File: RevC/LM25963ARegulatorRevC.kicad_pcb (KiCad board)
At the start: 2 copper layers, 61.2 x 24.6 mm, 18 parts, among them U1 LM2596S-ADJ

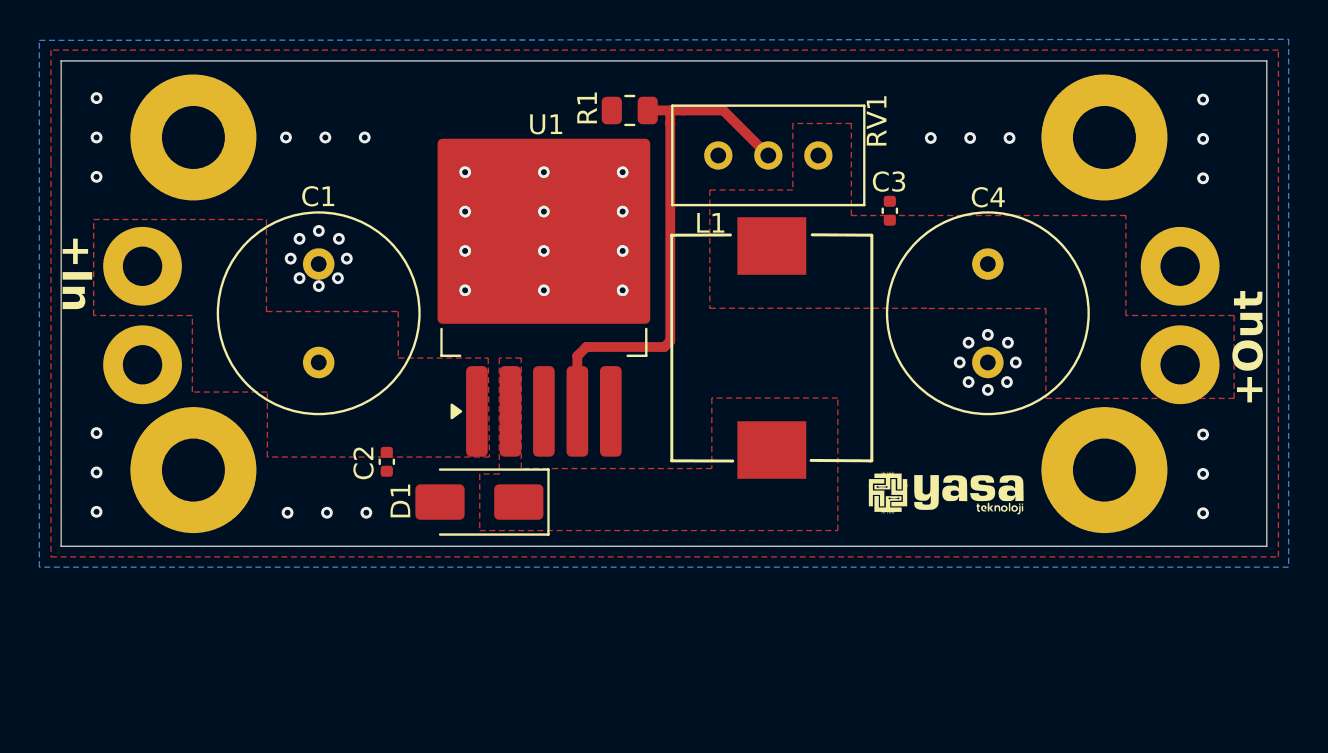
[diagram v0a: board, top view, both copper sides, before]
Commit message: Add files via upload
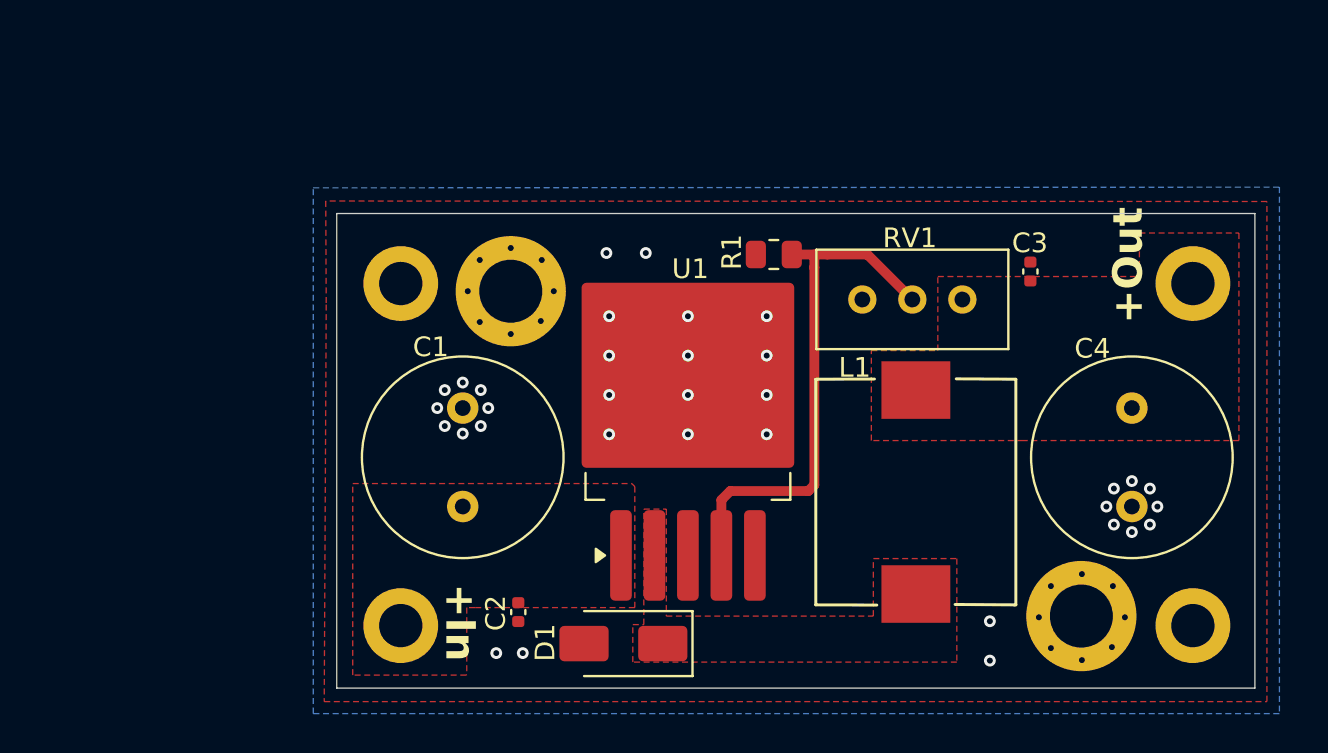
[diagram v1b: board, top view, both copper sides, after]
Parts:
- removed the ? at (121.1, 107.9)
- removed the ? at (167.4, 91.0)
- removed the ? at (167.4, 107.9)
- removed the ? at (171.3, 97.5)
- removed the ? at (171.3, 102.5)
- removed the REF** at (121.1, 91.0)
- removed the REF** at (118.6, 97.5)
- removed the REF** at (118.6, 102.5)
- added ?: , , F.Cu at (137.3, 98.8)
- added ?: , , F.Cu at (171.9, 98.4)
- added ?: , , F.Cu at (131.7, 98.4)
- added ?: , , F.Cu at (171.9, 115.8)
- added REF**: MountingHole_2.2mm_M2_DIN965_Pad, MountingHole:MountingHole_2.2mm_M2_DIN965_Pad, F.Cu at (131.7, 115.8)
- added REF**: MountingHole_3.2mm_M3_DIN965_Pad, MountingHole:MountingHole_3.2mm_M3_DIN965_Pad, F.Cu at (166.2, 115.3)
- G***: moved to B.Cu
- moved U1 10.3 mm to (146.3, 104.6)
- moved C1 10.3 mm to (134.8, 109.8)
- moved C4 10.3 mm to (168.8, 104.8)
- moved R1 10.3 mm to (150.6, 97.0)
- moved RV1 10.3 mm to (155.1, 99.2)
- moved L1 10.3 mm to (157.8, 109.0)
- moved D1 10.3 mm to (143.0, 116.7)
- moved C2 10.1 mm to (137.6, 115.1)
- moved G*** 8.23 mm to (151.1, 108.7)
- moved C3 7.78 mm to (163.7, 97.8)
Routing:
- net GND: vias 49 -> 50
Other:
- board size 61.2 x 24.6 mm -> 46.6 x 24.1 mm
